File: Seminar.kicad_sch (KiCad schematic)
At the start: 28 parts, among them SW1 SW_Push, SW2 SW_Push, SW3 SW_Nidec_CAS-120A1, U1 NUCLEO64-F446RE, U2 PCF8574AP, U4 TP4056-42-ESOP8

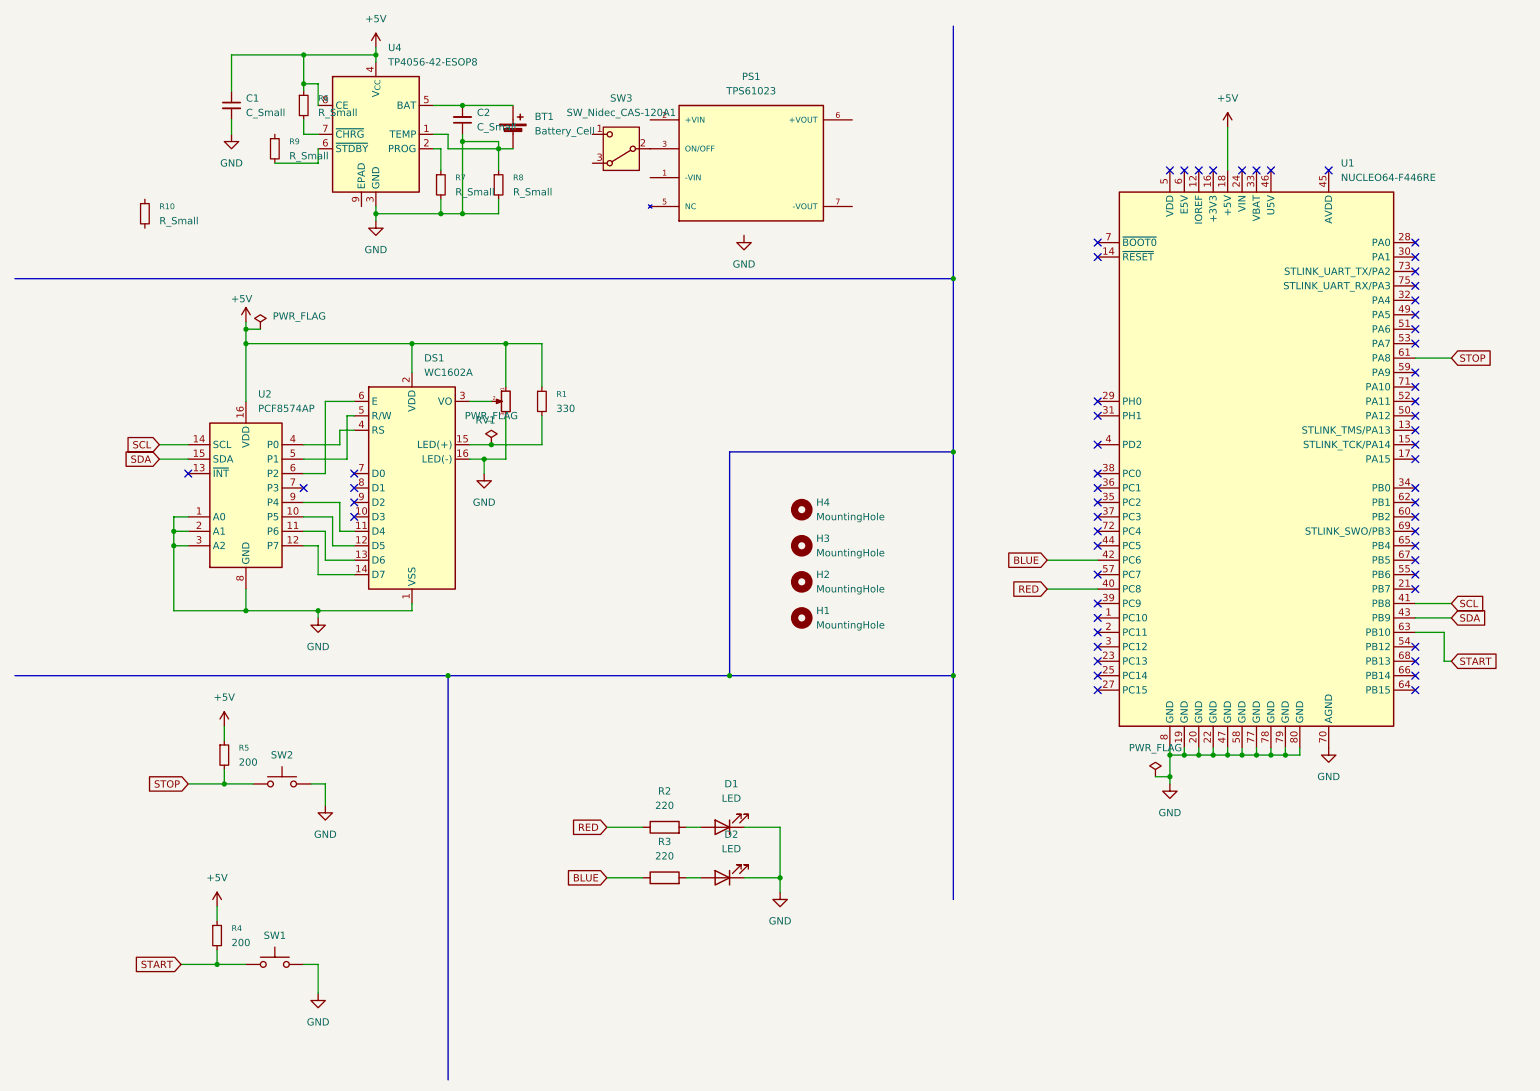
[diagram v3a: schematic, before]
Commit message: Mucenje
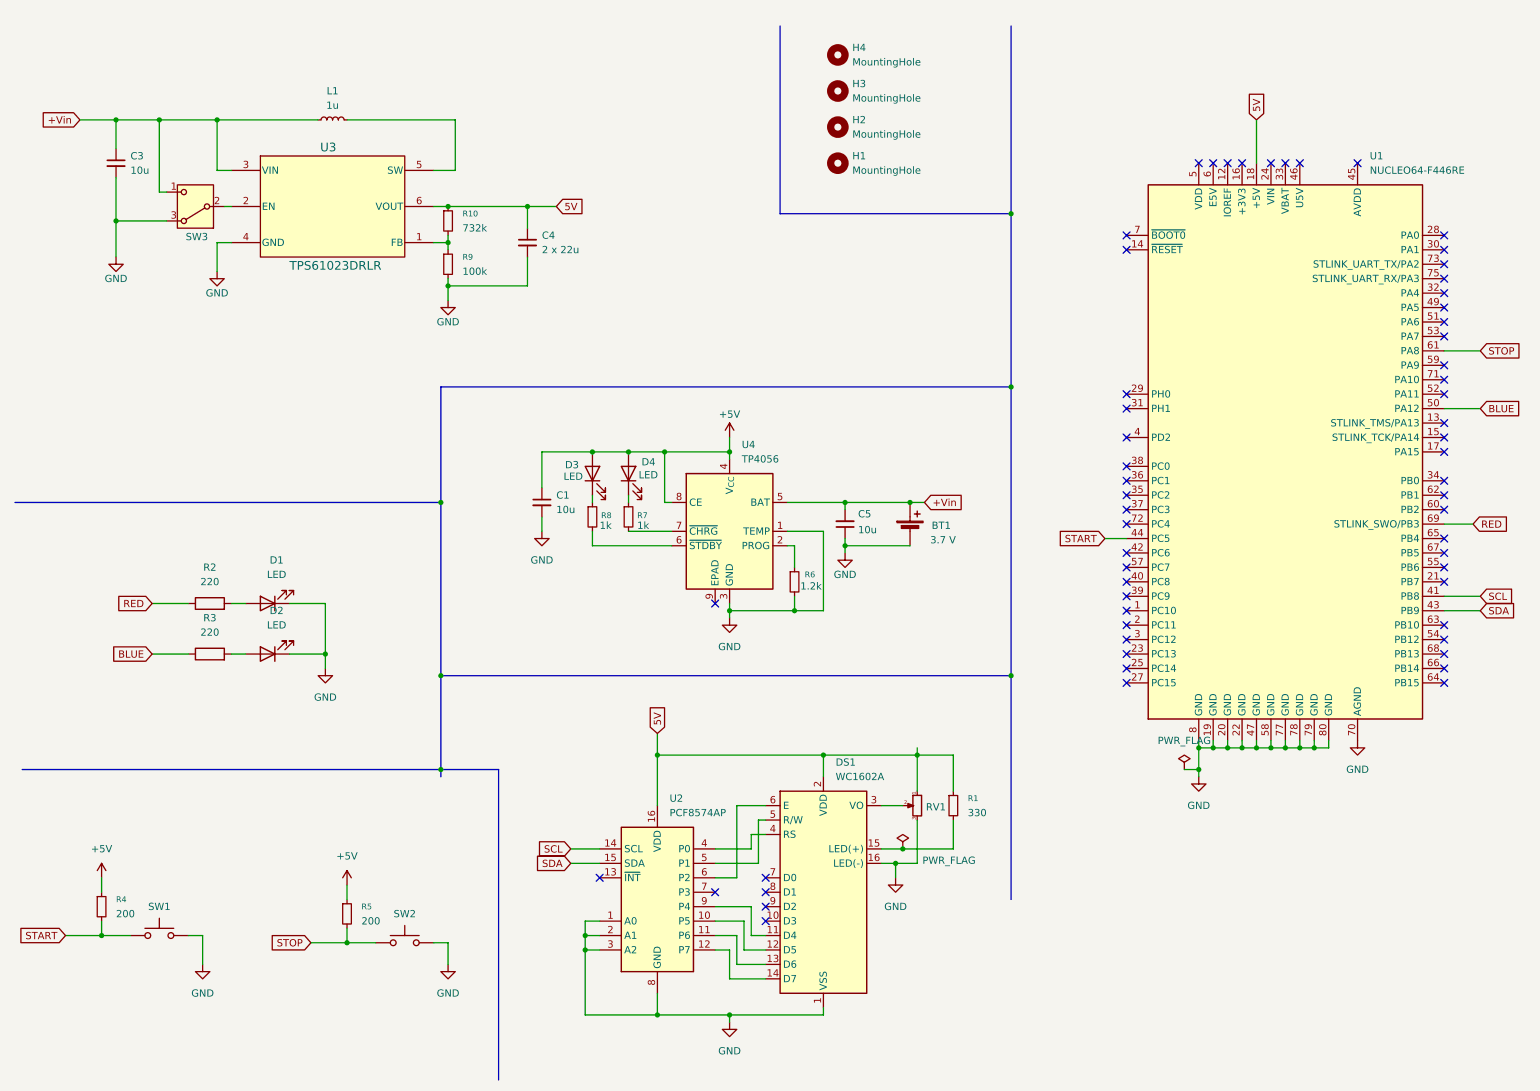
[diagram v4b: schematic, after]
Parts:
- removed PS1: TPS61023, CONV_PDQ2-D5-S3-S:CONV_PDQ2-D5-S3-S, symbol PDQ2-D5-S3-S:PDQ2-D5-S3-S
- removed R8: R_Small, symbol Device:R_Small
- added C3: 10u, Capacitor_SMD:C_1206_3216Metric_Pad1.33x1.80mm_HandSolder, symbol Device:C_Small
- added C4: 2 x 22u, Capacitor_THT:CP_Radial_D5.0mm_P2.00mm, symbol Device:C_Small
- added D3, D4: LED, LED_THT:LED_D5.0mm, symbol Device:LED
- added L1: 1u, Inductor_THT:L_Radial_D7.2mm_P3.00mm_Murata_1700, symbol Device:L_Small
- added R9: 100k, Resistor_SMD:R_1206_3216Metric_Pad1.30x1.75mm_HandSolder, symbol Device:R_Small
- added U3: TPS61023DRLR, footprints:DRL0006A, symbol 2025-12-11_16-22-03:TPS61023DRLR
- BT1: value Battery_Cell -> 3.7 V; footprint (none) -> Battery:BatteryHolder_Keystone_1042_1x18650; Manufacturer (none) -> EEMB; Manufacturer part number (none) -> LIR18650
- C1: value C_Small -> 10u; footprint (none) -> Capacitor_SMD:C_1206_3216Metric_Pad1.33x1.80mm_HandSolder; Manufacturer (none) -> SAMSUNG; Manufacturer part number (none) -> CL31A106KBHNNNE
- C5: renamed from C2; value C_Small -> 10u; footprint (none) -> Capacitor_SMD:C_1206_3216Metric_Pad1.33x1.80mm_HandSolder; Manufacturer (none) -> SAMSUNG; Manufacturer part number (none) -> CL31A106KBHNNNE
- R10: value R_Small -> 732k; footprint (none) -> Resistor_SMD:R_1206_3216Metric_Pad1.30x1.75mm_HandSolder; Manufacturer (none) -> ROYALOHM; Manufacturer part number (none) -> 1206S4J0473T5E
- R6: renamed from R7; value R_Small -> 1.2k; footprint (none) -> Resistor_SMD:R_1206_3216Metric_Pad1.30x1.75mm_HandSolder; Manufacturer (none) -> ROYALOHM; Manufacturer part number (none) -> 1206S4F2001T5E
- R7: renamed from R6; value R_Small -> 1k; footprint (none) -> Resistor_SMD:R_1206_3216Metric_Pad1.30x1.75mm_HandSolder; Manufacturer (none) -> ROYALOHM; Manufacturer part number (none) -> 1206S4F2001T5E
- R8: renamed from R9; value R_Small -> 1k; footprint (none) -> Resistor_SMD:R_1206_3216Metric_Pad1.30x1.75mm_HandSolder; Manufacturer (none) -> ROYALOHM; Manufacturer part number (none) -> 1206S4F2001T5E
- SW3: value SW_Nidec_CAS-120A1 -> ~
- U4: value TP4056-42-ESOP8 -> TP4056
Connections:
- net +5V: now also D3.2 (A), D4.2 (A); no longer DS1.2 (VDD), R1.1, R7.1, RV1.1, U1.18 (+5V), U2.16 (VDD)
- net BLUE: now also U1.50 (PA12); no longer U1.42 (PC6)
- net GND: now also SW3.3 (A), C3.2, C4.2, R9.2, U3.4 (GND)
- net RED: now also U1.69 (STLINK_SWO/PB3); no longer U1.40 (PC8)
- net START: now also U1.44 (PC5); no longer U1.63 (PB10)
- net +Vin: now reaches BT1.1 (+), C5.2, U4.5 (BAT)
- net +Vin: now also SW3.1 (C), C3.1, L1.1, U3.3 (VIN)
- net 5V: now reaches R10.1
- net 5V: now also DS1.2 (VDD), R1.1, RV1.1, U1.18 (+5V), U2.16 (VDD), C4.1, U3.6 (VOUT)
- net at R10.2: now also R9.1, U3.1 (FB)
- net at SW3.2 (B): now also U3.2 (EN)
- net at R8.1: now also D3.1 (K)
- new net: L1.2, U3.5 (SW)
- new net: D4.1 (K), R7.1
- no-connect marks 60 -> 61
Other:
- moved on the sheet: BT1, C1, C5, D1, D2, DS1, H1, H2, H3, H4, R1, R2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
